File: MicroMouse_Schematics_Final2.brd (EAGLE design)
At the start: 227 x 80 mm, 64 parts

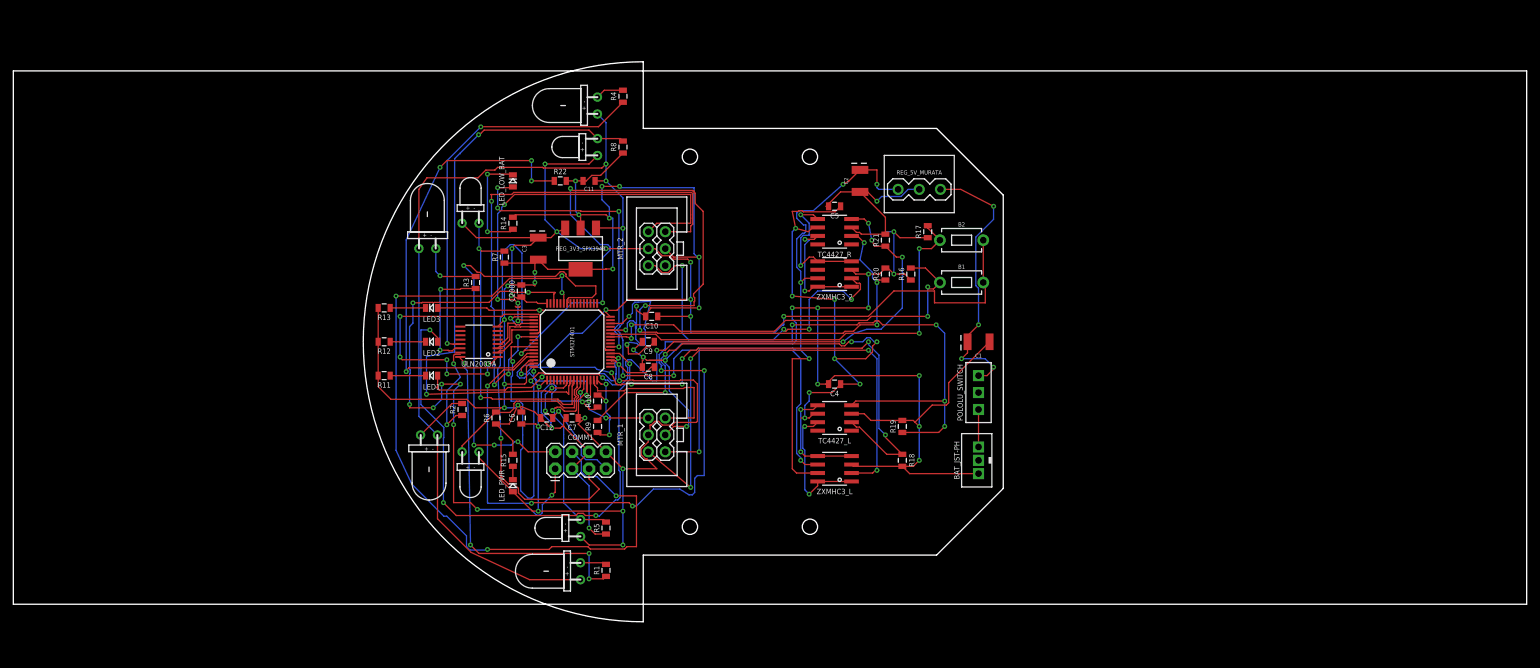
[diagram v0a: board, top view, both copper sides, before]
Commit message: Fixed error
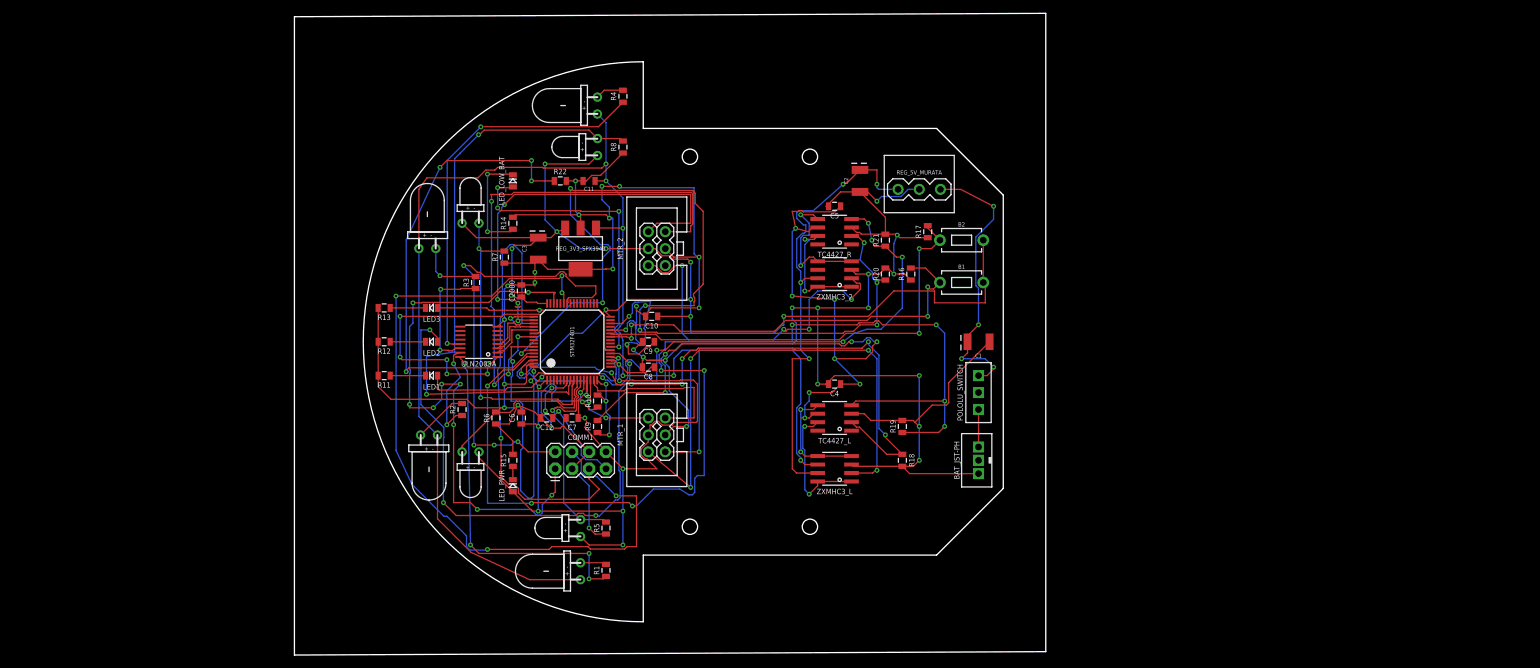
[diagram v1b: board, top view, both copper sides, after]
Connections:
- net +3V3: no longer C7.1
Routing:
- net +3V3: track 336.9 -> 336.0 mm
- net GND: track 214.8 -> 214.2 mm
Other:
- board size 227 x 80 mm -> 112.7 x 96.3 mm
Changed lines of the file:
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@@
 <?xml version="1.0" encoding="utf-8"?>
 <!DOCTYPE eagle SYSTEM "eagle.dtd">
-<eagle version="8.6.0">
+<eagle version="8.7.0">
 <drawing>
 <settings>
@@
 <board>
 <plain>
-<wire x1="0" y1="0" x2="227" y2="0" width="0" layer="20"/>
-<wire x1="227" y1="0" x2="227" y2="80" width="0" layer="20"/>
-<wire x1="227" y1="80" x2="0" y2="80" width="0" layer="20"/>
-<wire x1="0" y1="80" x2="0" y2="0" width="0" layer="20"/>
+<wire x1="42.164" y1="-7.62" x2="154.864" y2="-7.112" width="0" layer="20"/>
+<wire x1="154.864" y1="-7.112" x2="154.864" y2="88.636" width="0" layer="20"/>
+<wire x1="154.864" y1="88.636" x2="42.164" y2="88.128" width="0" layer="20"/>
+<wire x1="42.164" y1="88.128" x2="42.164" y2="-7.62" width="0" layer="20"/>
 </plain>
 <attributes>
@@
 <wire x1="132.08" y1="49.53" x2="133.72" y2="49.53" width="0.1524" layer="1"/>
 <wire x1="133.72" y1="49.53" x2="134.62" y2="48.63" width="0.1524" layer="1"/>
-<wire x1="132.08" y1="49.53" x2="132.08" y2="55.88" width="0.1524" layer="16"/>
-<via x="132.08" y="55.88" extent="1-16" drill="0.35"/>
-<wire x1="130.81" y1="55.88" x2="132.08" y2="55.88" width="0.1524" layer="16"/>
-<wire x1="132.08" y1="55.88" x2="132.98" y2="54.98" width="0.1524" layer="1"/>
+<wire x1="132.08" y1="49.53" x2="132.08" y2="54.102" width="0.1524" layer="16"/>
+<via x="132.588" y="55.372" extent="1-16" drill="0.35"/>
+<wire x1="132.08" y1="54.102" x2="132.588" y2="55.372" width="0.1524" layer="16"/>
+<wire x1="132.588" y1="55.372" x2="132.98" y2="54.98" width="0.1524" layer="1"/>
 <wire x1="132.98" y1="54.98" x2="137.16" y2="54.98" width="0.1524" layer="1"/>
 <wire x1="126.4666" y1="55.7784" x2="126.9295875" y2="55.7784" width="0.1524" layer="1"/>
@@
 <wire x1="94.488" y1="37.084" x2="94.9876" y2="36.5844" width="0.1524" layer="1"/>
 <wire x1="94.9876" y1="36.5844" x2="97.79" y2="36.5844" width="0.1524" layer="1"/>
-<wire x1="130.81" y1="55.88" x2="130.81" y2="55.51" width="0" layer="19" extent="1-16"/>
+<wire x1="130.81" y1="55.51" x2="132.45" y2="55.51" width="0.1524" layer="1"/>
+<wire x1="132.45" y1="55.51" x2="132.588" y2="55.372" width="0.1524" layer="1"/>
 </signal>
 <signal name="+5V">
@@
 <contactref element="STM32F401" pad="VBAT"/>
 <contactref element="C6" pad="1"/>
-<contactref element="C7" pad="1"/>
 <contactref element="STM32F401" pad="VDDA"/>
 <contactref element="STM32F401" pad="VDD_2"/>
@@
 <wire x1="78.74" y1="26.67" x2="78.37" y2="27.04" width="0.1524" layer="1"/>
 <wire x1="78.37" y1="27.04" x2="76.2" y2="27.04" width="0.1524" layer="1"/>
-<wire x1="88.9" y1="22.86" x2="84.72" y2="27.04" width="0.1524" layer="1"/>
-<wire x1="84.72" y1="27.04" x2="85.736" y2="27.94" width="0.1524" layer="1"/>
+<wire x1="88.9" y1="22.86" x2="85.736" y2="26.532" width="0.1524" layer="1"/>
+<wire x1="85.736" y1="26.532" x2="85.995565625" y2="27.26993125" width="0.1524" layer="1"/>
 <via x="85.736" y="27.94" extent="1-16" drill="0.35"/>
+<wire x1="85.995565625" y1="27.26993125" x2="85.736" y2="27.94" width="0.1524" layer="1"/>
 <wire x1="78.74" y1="54.99" x2="69.47" y2="54.99" width="0.1524" layer="1"/>
 <wire x1="69.47" y1="54.99" x2="67.31" y2="57.15" width="0.1524" layer="1"/>
@@
 <wire x1="145.49" y1="48.26" x2="145.49" y2="54.304" width="0.1524" layer="1"/>
 <wire x1="145.49" y1="54.304" x2="145.796" y2="54.61" width="0.1524" layer="1"/>
-<wire x1="84.7607125" y1="27.9807125" x2="84.72" y2="27.94" width="0" layer="19" extent="1-1"/>
 </signal>
 <signal name="N$4">
@@
 <wire x1="81.07" y1="46.526" x2="81.07" y2="45.12" width="0.1524" layer="1"/>
 <wire x1="63.1433125" y1="45.2786" x2="63.0094" y2="45.1446875" width="0.1524" layer="1"/>
-<wire x1="71.34445" y1="45.2786" x2="64.008" y2="45.2786" width="0.1524" layer="1"/>
-<wire x1="64.008" y1="45.2786" x2="63.1433125" y2="45.2786" width="0.1524" layer="1"/>
+<wire x1="71.34445" y1="45.2786" x2="63.1433125" y2="45.2786" width="0.1524" layer="1"/>
 <wire x1="74.92735" y1="46.9336" x2="72.99945" y2="46.9336" width="0.1524" layer="1"/>
 <wire x1="72.99945" y1="46.9336" x2="71.34445" y2="45.2786" width="0.1524" layer="1"/>
@@
 <wire x1="75.08425" y1="42.26185" x2="75.08425" y2="42.38235" width="0.1524" layer="16"/>
 <wire x1="75.08425" y1="42.38235" x2="74.5748" y2="42.8918" width="0.1524" layer="16"/>
-<wire x1="73.0532" y1="35.81665" x2="73.0532" y2="42.164" width="0.1524" layer="16"/>
-<wire x1="73.0532" y1="42.164" x2="73.0532" y2="42.93695" width="0.1524" layer="16"/>
+<wire x1="73.0532" y1="35.81665" x2="73.0532" y2="42.93695" width="0.1524" layer="16"/>
 <wire x1="73.0532" y1="42.93695" x2="73.3612" y2="43.24495" width="0.1524" layer="16"/>
 <wire x1="73.3612" y1="43.24495" x2="73.3612" y2="52.76875" width="0.1524" layer="16"/>
 <wire x1="73.3612" y1="52.76875" x2="74.53925" y2="53.9468" width="0.1524" layer="16"/>
 <wire x1="75.04195" y1="53.9468" x2="76.2988" y2="52.68995" width="0.1524" layer="16"/>
-<wire x1="76.2988" y1="52.68995" x2="76.2988" y2="43.18" width="0.1524" layer="16"/>
-<wire x1="76.2988" y1="43.18" x2="76.2988" y2="42.2628" width="0.1524" layer="16"/>
+<wire x1="76.2988" y1="52.68995" x2="76.2988" y2="42.2628" width="0.1524" layer="16"/>
 </signal>
 <signal name="NRST">
@@
 <wire x1="74.6932" y1="30.4628" x2="75.94335" y2="30.4628" width="0.1524" layer="16"/>
 <wire x1="75.94335" y1="30.4628" x2="76.4032" y2="30.00295" width="0.1524" layer="16"/>
-<wire x1="76.4032" y1="30.00295" x2="76.4032" y2="25.4" width="0.1524" layer="16"/>
-<wire x1="76.4032" y1="25.4" x2="76.4032" y2="23.41335" width="0.1524" layer="16"/>
+<wire x1="76.4032" y1="30.00295" x2="76.4032" y2="23.41335" width="0.1524" layer="16"/>
 <wire x1="78.0768" y1="33.02" x2="77.681303125" y2="33.415496875" width="0.1524" layer="16"/>
 <wire x1="77.681303125" y1="33.415496875" x2="77.681303125" y2="33.5707" width="0.1524" layer="16"/>
@@
 <wire x1="79.547425" y1="34.690875" x2="78.801478125" y2="34.690875" width="0.1524" layer="1"/>
 <wire x1="78.801478125" y1="34.690875" x2="77.625203125" y2="33.5146" width="0.1524" layer="1"/>
-<wire x1="78.07" y1="38.62" x2="75.184" y2="38.62" width="0.1524" layer="1"/>
-<wire x1="75.184" y1="38.62" x2="74.688" y2="38.62" width="0.1524" layer="1"/>
+<wire x1="78.07" y1="38.62" x2="74.688" y2="38.62" width="0.1524" layer="1"/>
 <wire x1="74.688" y1="38.62" x2="74.676" y2="38.608" width="0.1524" layer="1"/>
 <wire x1="74.688" y1="38.62" x2="74.688" y2="36.63344375" width="0.1524" layer="1"/>
@@
 <wire x1="95.25" y1="55.88" x2="96.52" y2="57.15" width="0.1524" layer="1"/>
 <wire x1="96.52" y1="57.15" x2="101.6" y2="57.15" width="0.1524" layer="1"/>
-<wire x1="101.6" y1="57.15" x2="101.6" y2="57.912" width="0.1524" layer="1"/>
-<wire x1="101.6" y1="57.912" x2="101.6" y2="58.42" width="0.1524" layer="1"/>
 <wire x1="78.07" y1="42.62" x2="76.252" y2="42.62" width="0.1524" layer="1"/>
 <wire x1="76.252" y1="42.62" x2="76.2" y2="42.672" width="0.1524" layer="1"/>
@@
 <wire x1="73.66" y1="59.944" x2="75.184" y2="61.468" width="0.1524" layer="1"/>
 <wire x1="75.184" y1="61.468" x2="101.6" y2="61.468" width="0.1524" layer="1"/>
-<wire x1="101.6" y1="61.468" x2="101.6" y2="58.42" width="0.1524" layer="1"/>
+<wire x1="101.6" y1="61.468" x2="101.6" y2="57.15" width="0.1524" layer="1"/>
 </signal>
 <signal name="RMTR-">
@@
 <wire x1="66.04" y1="36.068" x2="66.04" y2="37.3332875" width="0.1524" layer="1"/>
 <wire x1="66.04" y1="37.3332875" x2="66.1999125" y2="37.4932" width="0.1524" layer="1"/>
-<wire x1="66.1999125" y1="37.4932" x2="67.05" y2="37.4932" width="0.1524" layer="1"/>
-<wire x1="67.05" y1="37.4932" x2="67.05" y2="37.745" width="0" layer="19" extent="1-1"/>
+<wire x1="66.1999125" y1="37.4932" x2="66.548" y2="37.592" width="0.1524" layer="1"/>
+<wire x1="66.548" y1="37.592" x2="67.056" y2="37.739" width="0.1524" layer="1"/>
+<wire x1="67.056" y1="37.739" x2="67.05" y2="37.745" width="0.1524" layer="1"/>
 </signal>
 <signal name="N$11">
@@
 <contactref element="ULN2003A" pad="4C"/>
 <contactref element="R4" pad="1"/>
-<wire x1="91.44" y1="75.3" x2="88.08" y2="71.94" width="0.1524" layer="1"/>
-<wire x1="88.08" y1="71.94" x2="87.768" y2="71.628" width="0.1524" layer="1"/>
+<wire x1="91.44" y1="75.3" x2="87.768" y2="71.628" width="0.1524" layer="1"/>
 <wire x1="87.768" y1="71.628" x2="70.104" y2="71.628" width="0.1524" layer="1"/>
 <wire x1="70.104" y1="71.628" x2="70.11743125" y2="71.61456875" width="0.1524" layer="1"/>
@@
 <wire x1="88.53" y1="12.7" x2="85.09" y2="12.7" width="0.1524" layer="1"/>
 <wire x1="85.09" y1="12.7" x2="82.55" y2="15.24" width="0.1524" layer="16"/>
-<wire x1="82.55" y1="15.24" x2="82.55" y2="24.892" width="0.1524" layer="16"/>
-<wire x1="82.55" y1="24.892" x2="82.55" y2="25.4" width="0.1524" layer="16"/>
+<wire x1="82.55" y1="15.24" x2="82.55" y2="26.722953125" width="0.1524" layer="16"/>
 <wire x1="84.46193125" y1="32.02261875" x2="84.46193125" y2="31.51991875" width="0.1524" layer="1"/>
 <wire x1="85.07" y1="33.62" x2="85.07" y2="32.6306875" width="0.1524" layer="1"/>
@@
 <via x="80.8792" y="29.0706" extent="1-16" drill="0.35"/>
 <wire x1="80.8792" y1="29.0706" x2="81.1812" y2="28.7686" width="0.1524" layer="16"/>
-<wire x1="82.55" y1="26.722953125" x2="82.55" y2="25.4" width="0.1524" layer="16"/>
 <wire x1="81.1812" y1="28.7686" x2="81.1812" y2="28.091753125" width="0.1524" layer="16"/>
 <wire x1="81.1812" y1="28.091753125" x2="82.55" y2="26.722953125" width="0.1524" layer="16"/>
@@
 <wire x1="70.104" y1="30.988" x2="70.104" y2="53.086" width="0.1524" layer="16"/>
 <wire x1="70.104" y1="53.086" x2="69.85" y2="53.34" width="0.1524" layer="16"/>
-<wire x1="81.6966625" y1="30.7676" x2="73.152" y2="30.7676" width="0.1524" layer="1"/>
-<wire x1="73.152" y1="30.7676" x2="71.8484" y2="30.7676" width="0.1524" layer="1"/>
+<wire x1="81.6966625" y1="30.7676" x2="71.8484" y2="30.7676" width="0.1524" layer="1"/>
 </signal>
 <signal name="RE_RF">
